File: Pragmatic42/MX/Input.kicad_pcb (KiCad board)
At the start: 2 copper layers, 127.2 x 85.4 mm, 90 parts, among them J1 Conn_02x04_Odd_Even, SW13 SW_Push_45deg, SW14 SW_Push_45deg, SW15 SW_Push_45deg, SW16 SW_Push_45deg, SW17 SW_Push_45deg, SW18 SW_Push_45deg, SW19 SW_Push_45deg, SW20 SW_Push_45deg, SW21 SW_Push_45deg, SW22 SW_Push_45deg, SW23 SW_Push_45deg, SW24 SW_Push_45deg, SW25 SW_Push_45deg, SW26 SW_Push_45deg, SW27 SW_Push_45deg, SW28 SW_Push_45deg, SW29 SW_Push_45deg, SW30 SW_Push_45deg, SW31 SW_Push_45deg, SW32 SW_Push_45deg, SW33 SW_Push_45deg, SW34 SW_Push_45deg, SW35 SW_Push_45deg, SW36 SW_Push_45deg, SW37 SW_Push_45deg, SW38 SW_Push_45deg, SW39 SW_Push_45deg, SW40 SW_Push_45deg, SW41 SW_Push_45deg, SW42 SW_Push_45deg, SW43 SW_Push_45deg, SW44 SW_Push_45deg, SW45 SW_Push_45deg, SW46 SW_Push_45deg, SW47 SW_Push_45deg, SW48 SW_Push_45deg, SW52 SW_Push_45deg, SW53 SW_Push_45deg, SW54 SW_Push_45deg, SW55 SW_Push_45deg, SW56 SW_Push_45deg, SW57 SW_Push_45deg

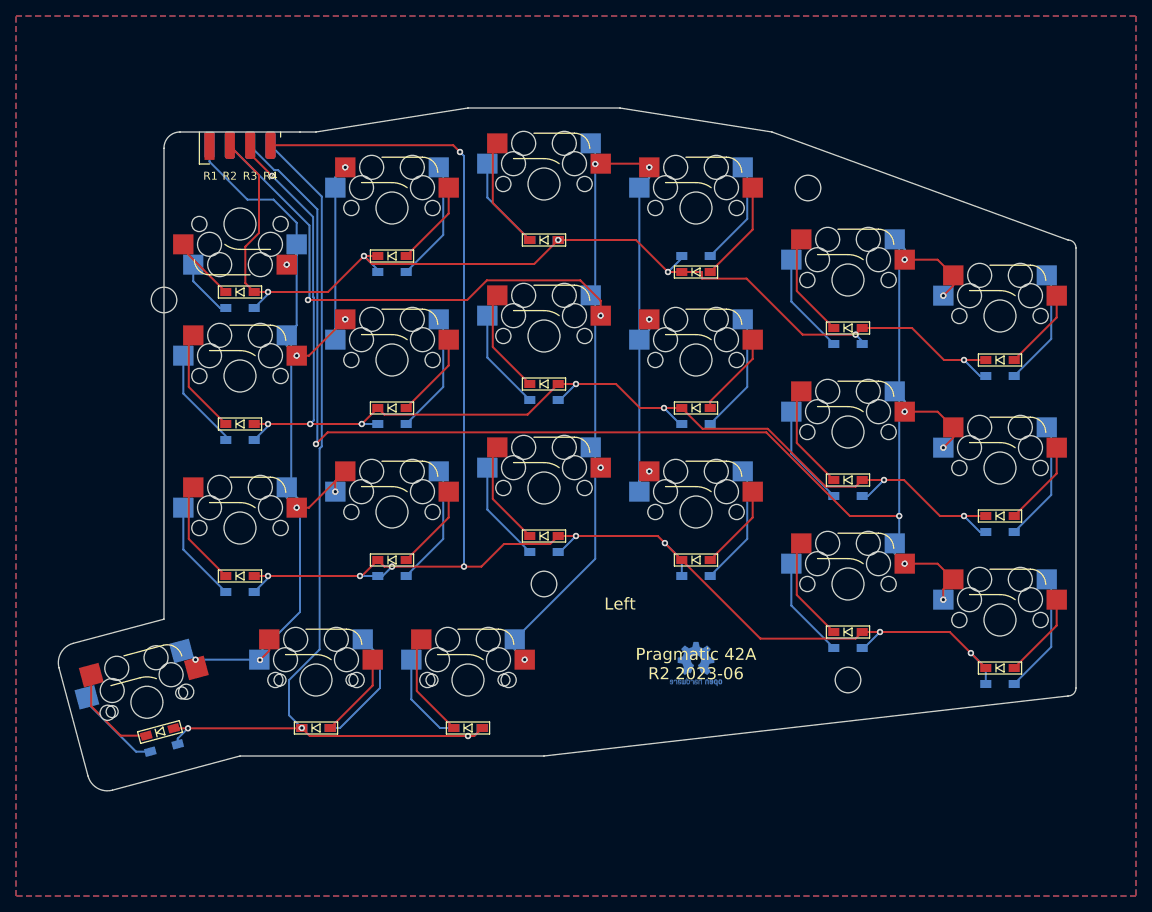
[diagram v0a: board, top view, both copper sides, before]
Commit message: placement
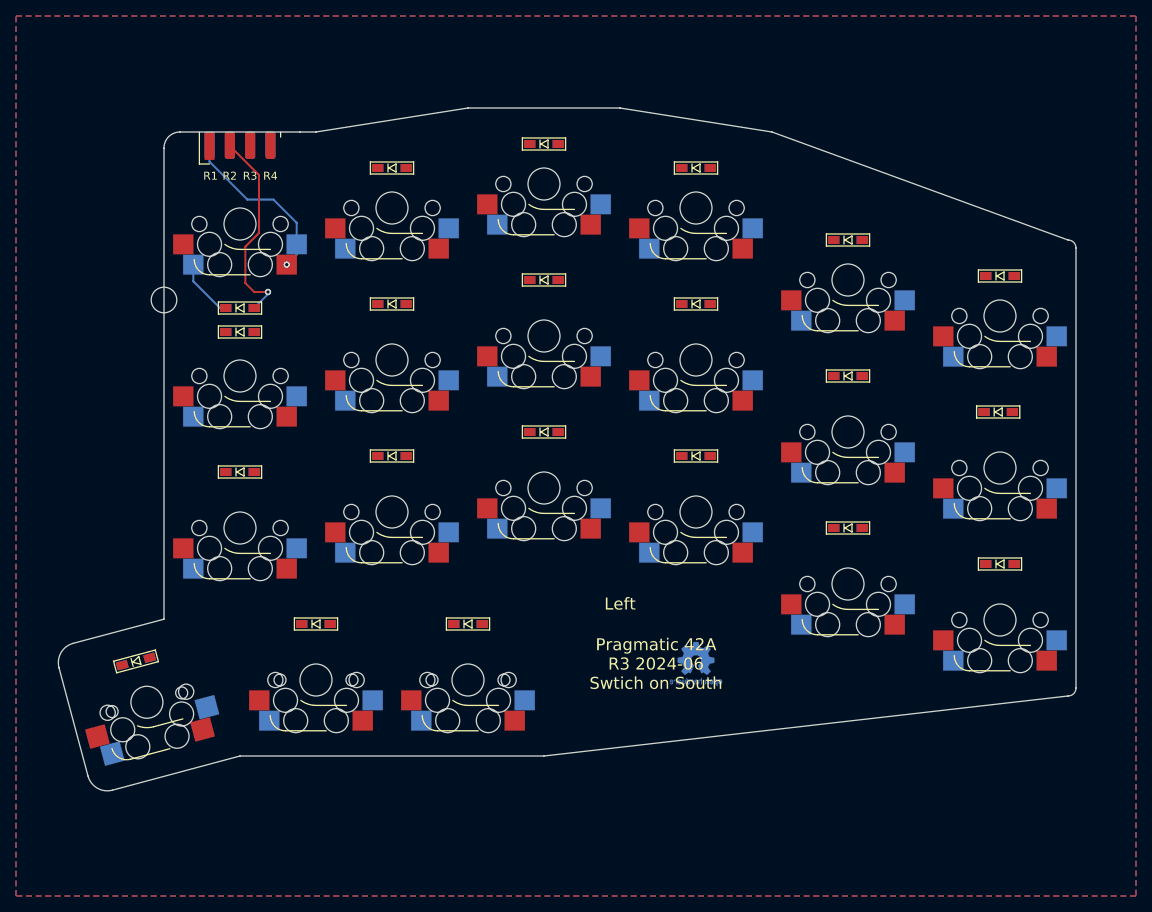
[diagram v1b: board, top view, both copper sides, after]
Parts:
- removed H1, H2, H3: MountingHole, MountingHole:MountingHole_3.2mm_M3_DIN965
- moved D36 15.0 mm to (213.8, 97.5)
- moved D32 15.0 mm to (138.0, 84.0)
- moved D33 15.0 mm to (157.0, 81.0)
- moved D34 15.0 mm to (176.0, 84.0)
- moved D35 15.0 mm to (195.0, 93.0)
- moved D43 15.0 mm to (119.0, 105.0)
- moved D44 15.0 mm to (138.0, 103.0)
- moved D45 15.0 mm to (157.0, 100.0)
- moved D46 15.0 mm to (176.0, 103.0)
- moved D47 15.0 mm to (195.0, 112.0)
- moved D48 15.0 mm to (214.0, 116.5)
- moved D31 13.5 mm to (119.0, 87.5)
- moved D25 13.0 mm to (213.8, 97.5)
- moved D53 13.0 mm to (128.5, 124.0)
- moved D56 13.0 mm to (128.5, 124.0)
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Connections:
- SW13 pad 1: C56 -> Net-(D13-A)
- SW13 pad 2: Net-(D13-A) -> C56
- SW14 pad 1: Net-(D14-K) -> C56
- SW14 pad 2: C56 -> Net-(D14-K)
- SW15 pad 1: C34 -> Net-(D15-A)
- SW15 pad 2: Net-(D15-A) -> C34
- SW16 pad 1: Net-(D16-K) -> C34
- SW16 pad 2: C34 -> Net-(D16-K)
- SW17 pad 1: C12 -> Net-(D17-A)
- SW17 pad 2: Net-(D17-A) -> C12
- SW20 pad 1: C12 -> Net-(D20-K)
- SW20 pad 2: Net-(D20-K) -> C12
- SW21 pad 1: Net-(D21-A) -> C34
- SW21 pad 2: C34 -> Net-(D21-A)
- SW22 pad 1: C34 -> Net-(D22-K)
- SW22 pad 2: Net-(D22-K) -> C34
- SW23 pad 1: Net-(D23-A) -> C56
- SW23 pad 2: C56 -> Net-(D23-A)
- SW24 pad 1: C56 -> Net-(D24-K)
- SW24 pad 2: Net-(D24-K) -> C56
- SW25 pad 1: C56 -> Net-(D25-A)
- SW25 pad 2: Net-(D25-A) -> C56
- SW26 pad 1: Net-(D26-K) -> C56
- SW26 pad 2: C56 -> Net-(D26-K)
- SW27 pad 1: C34 -> Net-(D27-A)
- SW27 pad 2: Net-(D27-A) -> C34
- SW28 pad 1: Net-(D28-K) -> C34
- SW28 pad 2: C34 -> Net-(D28-K)
- SW29 pad 1: C12 -> Net-(D29-A)
- SW29 pad 2: Net-(D29-A) -> C12
- SW30 pad 1: Net-(D30-K) -> C12
- SW30 pad 2: C12 -> Net-(D30-K)
- SW31 pad 1: Net-(D31-A) -> C12
- SW31 pad 2: C12 -> Net-(D31-A)
- SW32 pad 1: C12 -> Net-(D32-K)
- SW32 pad 2: Net-(D32-K) -> C12
- SW33 pad 1: Net-(D33-A) -> C34
- SW33 pad 2: C34 -> Net-(D33-A)
- SW34 pad 1: C34 -> Net-(D34-K)
- SW34 pad 2: Net-(D34-K) -> C34
- SW35 pad 1: Net-(D35-A) -> C56
- SW35 pad 2: C56 -> Net-(D35-A)
- SW36 pad 1: C56 -> Net-(D36-K)
- SW36 pad 2: Net-(D36-K) -> C56
- SW37 pad 1: C56 -> Net-(D37-A)
- SW37 pad 2: Net-(D37-A) -> C56
- SW38 pad 1: Net-(D38-K) -> C56
- SW38 pad 2: C56 -> Net-(D38-K)
- SW39 pad 1: C34 -> Net-(D39-A)
- SW39 pad 2: Net-(D39-A) -> C34
- SW40 pad 1: Net-(D40-K) -> C34
- SW40 pad 2: C34 -> Net-(D40-K)
- SW41 pad 1: C12 -> Net-(D41-A)
- SW41 pad 2: Net-(D41-A) -> C12
- SW42 pad 1: Net-(D42-K) -> C12
- SW42 pad 2: C12 -> Net-(D42-K)
- SW43 pad 1: Net-(D43-A) -> C12
- SW43 pad 2: C12 -> Net-(D43-A)
- SW44 pad 1: C12 -> Net-(D44-K)
- SW44 pad 2: Net-(D44-K) -> C12
- SW45 pad 1: Net-(D45-A) -> C34
- SW45 pad 2: C34 -> Net-(D45-A)
- SW46 pad 1: C34 -> Net-(D46-K)
- SW46 pad 2: Net-(D46-K) -> C34
- SW47 pad 1: Net-(D47-A) -> C56
- SW47 pad 2: C56 -> Net-(D47-A)
- SW48 pad 1: C56 -> Net-(D48-K)
- SW48 pad 2: Net-(D48-K) -> C56
- SW52 pad 1: Net-(D52-K) -> C34
- SW52 pad 2: C34 -> Net-(D52-K)
- SW53 pad 1: C12 -> Net-(D53-A)
- SW53 pad 2: Net-(D53-A) -> C12
- SW54 pad 1: Net-(D54-K) -> C12
- SW54 pad 2: C12 -> Net-(D54-K)
- SW55 pad 1: Net-(D55-A) -> C12
- SW55 pad 2: C12 -> Net-(D55-A)
- SW56 pad 1: C12 -> Net-(D56-K)
- SW56 pad 2: Net-(D56-K) -> C12
- SW57 pad 1: Net-(D57-A) -> C34
- SW57 pad 2: C34 -> Net-(D57-A)
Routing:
- net Row 4: track 200.3 -> 0.00 mm, vias 9 -> 0
- net C56: track 193.7 -> 0.00 mm, vias 8 -> 0
- net C34: track 184.9 -> 0.00 mm, vias 8 -> 0
- net Row 3: track 156.4 -> 0.00 mm, vias 8 -> 0
- net Row 5: track 121.9 -> 0.00 mm, vias 3 -> 0
- net C12: track 138.7 -> 21.8 mm, vias 8 -> 1
- net Row 2: track 137.3 -> 25.4 mm, vias 6 -> 1
- net Net-(D56-K): track 15.3 -> 0.00 mm
- net Net-(D48-K): track 14.4 -> 0.00 mm
- net Net-(D46-K): track 14.4 -> 0.00 mm
- net Net-(D44-K): track 14.4 -> 0.00 mm
- net Net-(D36-K): track 14.4 -> 0.00 mm
- net Net-(D34-K): track 14.4 -> 0.00 mm
- net Net-(D32-K): track 14.4 -> 0.00 mm
- net Net-(D20-K): track 14.4 -> 0.00 mm
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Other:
- board text added: "Pragmatic 42A R3 2024-06 Swtich on South"
- board text removed: "Pragmatic 42A R2 2023-06"
